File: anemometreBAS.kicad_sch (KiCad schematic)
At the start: 12 parts, among them J1 Conn_01x03_Male, J2 Conn_01x02_Male, J3 Conn_01x02_Male, J4 Conn_01x02_Male, J5 Conn_01x02_Male, U1 TP4056

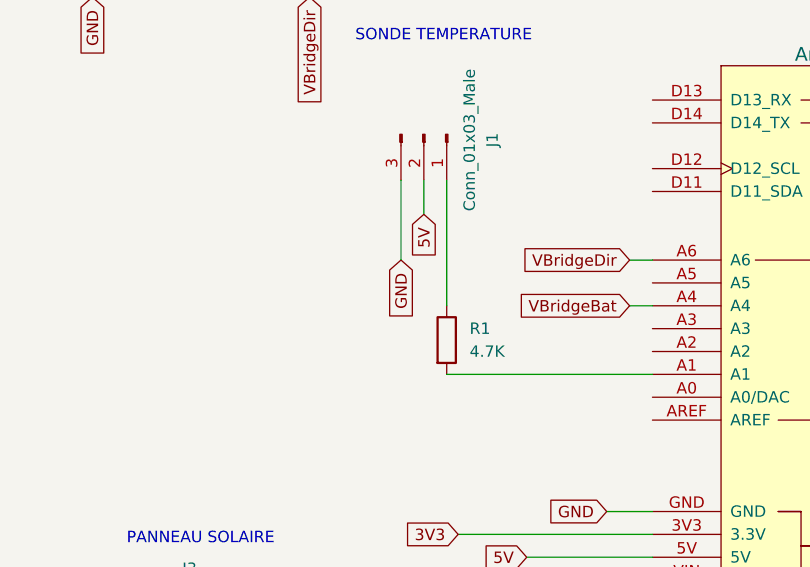
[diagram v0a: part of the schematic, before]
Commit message: fix error
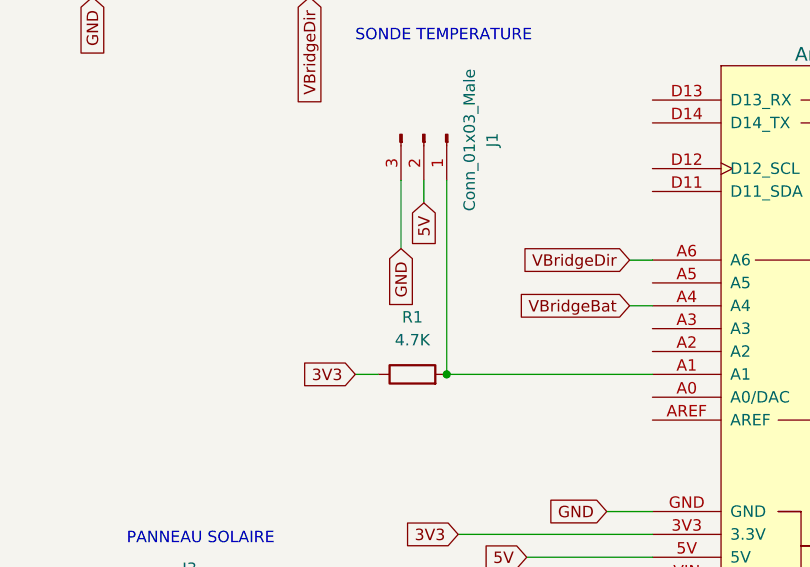
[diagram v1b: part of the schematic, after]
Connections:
- net 3V3: now also R1.1
- net at J1.1 (Pin_1): now also R1.2, XA1.A1; no longer R1.1
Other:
- moved on the sheet: R1
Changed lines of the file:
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@@
 (kicad_sch (version 20211123) (generator eeschema)
   (paper "A4")
+  (junction (at 100.33 86.36) (diameter 0) (color 0 0 0 0)
+  )
   (junction (at 34.29 76.2) (diameter 0) (color 0 0 0 0)
   )
@@
   (junction (at 199.39 55.88) (diameter 0) (color 0 0 0 0)
   )
+  (wire (pts (xy 90.17 86.36) (xy 92.71 86.36))
+    (stroke (width 0) (type default) (color 0 0 0 0))
+  )
+  (wire (pts (xy 199.39 55.88) (xy 208.28 55.88))
+    (stroke (width 0) (type default) (color 0 0 0 0))
+  )
+  (wire (pts (xy 76.2 113.03) (xy 83.82 113.03))
+    (stroke (width 0) (type default) (color 0 0 0 0))
+  )
+  (wire (pts (xy 34.29 60.96) (xy 34.29 66.04))
+    (stroke (width 0) (type default) (color 0 0 0 0))
+  )
+  (wire (pts (xy 205.74 58.42) (xy 208.28 58.42))
+    (stroke (width 0) (type default) (color 0 0 0 0))
+  )
+  (wire (pts (xy 34.29 76.2) (xy 38.1 76.2))
+    (stroke (width 0) (type default) (color 0 0 0 0))
+  )
+  (wire (pts (xy 118.11 109.22) (xy 123.19 109.22))
+    (stroke (width 0) (type default) (color 0 0 0 0))
+  )
+  (wire (pts (xy 34.29 86.36) (xy 34.29 91.44))
+    (stroke (width 0) (type default) (color 0 0 0 0))
+  )
+  (wire (pts (xy 101.6 104.14) (xy 123.19 104.14))
+    (stroke (width 0) (type default) (color 0 0 0 0))
+  )
+  (wire (pts (xy 76.2 115.57) (xy 83.82 115.57))
+    (stroke (width 0) (type default) (color 0 0 0 0))
+  )
+  (wire (pts (xy 120.65 78.74) (xy 123.19 78.74))
+    (stroke (width 0) (type default) (color 0 0 0 0))
+  )
+  (wire (pts (xy 80.01 125.73) (xy 83.82 125.73))
+    (stroke (width 0) (type default) (color 0 0 0 0))
+  )
+  (wire (pts (xy 97.79 64.77) (xy 97.79 67.31))
+    (stroke (width 0) (type default) (color 0 0 0 0))
+  )
+  (wire (pts (xy 120.65 73.66) (xy 123.19 73.66))
+    (stroke (width 0) (type default) (color 0 0 0 0))
+  )
+  (wire (pts (xy 189.23 55.88) (xy 199.39 55.88))
+    (stroke (width 0) (type default) (color 0 0 0 0))
+  )
+  (wire (pts (xy 60.96 40.64) (xy 60.96 44.45))
+    (stroke (width 0) (type default) (color 0 0 0 0))
+  )
+  (wire (pts (xy 199.39 40.64) (xy 199.39 48.26))
+    (stroke (width 0) (type default) (color 0 0 0 0))
+  )
+  (wire (pts (xy 72.39 128.27) (xy 83.82 128.27))
+    (stroke (width 0) (type default) (color 0 0 0 0))
+  )
+  (wire (pts (xy 109.22 106.68) (xy 123.19 106.68))
+    (stroke (width 0) (type default) (color 0 0 0 0))
+  )
+  (wire (pts (xy 85.09 40.64) (xy 85.09 38.1))
+    (stroke (width 0) (type default) (color 0 0 0 0))
+  )
+  (wire (pts (xy 95.25 64.77) (xy 95.25 72.39))
+    (stroke (width 0) (type default) (color 0 0 0 0))
+  )
+  (wire (pts (xy 60.96 120.65) (xy 83.82 120.65))
+    (stroke (width 0) (type default) (color 0 0 0 0))
+  )
+  (wire (pts (xy 118.11 101.6) (xy 123.19 101.6))
+    (stroke (width 0) (type default) (color 0 0 0 0))
+  )
+  (wire (pts (xy 85.09 40.64) (xy 85.09 44.45))
+    (stroke (width 0) (type default) (color 0 0 0 0))
+  )
+  (wire (pts (xy 60.96 118.11) (xy 83.82 118.11))
+    (stroke (width 0) (type default) (color 0 0 0 0))
+  )
+  (wire (pts (xy 34.29 73.66) (xy 34.29 76.2))
+    (stroke (width 0) (type default) (color 0 0 0 0))
+  )
+  (wire (pts (xy 34.29 76.2) (xy 34.29 78.74))
+    (stroke (width 0) (type default) (color 0 0 0 0))
+  )
+  (wire (pts (xy 63.5 40.64) (xy 85.09 40.64))
+    (stroke (width 0) (type default) (color 0 0 0 0))
+  )
+  (wire (pts (xy 85.09 25.4) (xy 85.09 30.48))
+    (stroke (width 0) (type default) (color 0 0 0 0))
+  )
+  (wire (pts (xy 100.33 64.77) (xy 100.33 86.36))
+    (stroke (width 0) (type default) (color 0 0 0 0))
+  )
   (wire (pts (xy 100.33 86.36) (xy 123.19 86.36))
-    (stroke (width 0) (type default) (color 0 0 0 0))
-  )
-  (wire (pts (xy 199.39 55.88) (xy 208.28 55.88))
-    (stroke (width 0) (type default) (color 0 0 0 0))
-  )
-  (wire (pts (xy 76.2 113.03) (xy 83.82 113.03))
-    (stroke (width 0) (type default) (color 0 0 0 0))
-  )
-  (wire (pts (xy 34.29 60.96) (xy 34.29 66.04))
-    (stroke (width 0) (type default) (color 0 0 0 0))
-  )
-  (wire (pts (xy 205.74 58.42) (xy 208.28 58.42))
-    (stroke (width 0) (type default) (color 0 0 0 0))
-  )
-  (wire (pts (xy 34.29 76.2) (xy 38.1 76.2))
-    (stroke (width 0) (type default) (color 0 0 0 0))
-  )
-  (wire (pts (xy 118.11 109.22) (xy 123.19 109.22))
-    (stroke (width 0) (type default) (color 0 0 0 0))
-  )
-  (wire (pts (xy 34.29 86.36) (xy 34.29 91.44))
-    (stroke (width 0) (type default) (color 0 0 0 0))
-  )
-  (wire (pts (xy 101.6 104.14) (xy 123.19 104.14))
-    (stroke (width 0) (type default) (color 0 0 0 0))
-  )
-  (wire (pts (xy 76.2 115.57) (xy 83.82 115.57))
-    (stroke (width 0) (type default) (color 0 0 0 0))
-  )
-  (wire (pts (xy 120.65 78.74) (xy 123.19 78.74))
-    (stroke (width 0) (type default) (color 0 0 0 0))
-  )
-  (wire (pts (xy 80.01 125.73) (xy 83.82 125.73))
-    (stroke (width 0) (type default) (color 0 0 0 0))
-  )
-  (wire (pts (xy 97.79 64.77) (xy 97.79 68.58))
-    (stroke (width 0) (type default) (color 0 0 0 0))
-  )
-  (wire (pts (xy 120.65 73.66) (xy 123.19 73.66))
-    (stroke (width 0) (type default) (color 0 0 0 0))
-  )
-  (wire (pts (xy 189.23 55.88) (xy 199.39 55.88))
-    (stroke (width 0) (type default) (color 0 0 0 0))
-  )
-  (wire (pts (xy 60.96 40.64) (xy 60.96 44.45))
-    (stroke (width 0) (type default) (color 0 0 0 0))
-  )
-  (wire (pts (xy 199.39 40.64) (xy 199.39 48.26))
-    (stroke (width 0) (type default) (color 0 0 0 0))
-  )
-  (wire (pts (xy 72.39 128.27) (xy 83.82 128.27))
-    (stroke (width 0) (type default) (color 0 0 0 0))
-  )
-  (wire (pts (xy 109.22 106.68) (xy 123.19 106.68))
-    (stroke (width 0) (type default) (color 0 0 0 0))
-  )
-  (wire (pts (xy 85.09 40.64) (xy 85.09 38.1))
-    (stroke (width 0) (type default) (color 0 0 0 0))
-  )
-  (wire (pts (xy 95.25 64.77) (xy 95.25 73.66))
-    (stroke (width 0) (type default) (color 0 0 0 0))
-  )
-  (wire (pts (xy 60.96 120.65) (xy 83.82 120.65))
-    (stroke (width 0) (type default) (color 0 0 0 0))
-  )
-  (wire (pts (xy 118.11 101.6) (xy 123.19 101.6))
-    (stroke (width 0) (type default) (color 0 0 0 0))
-  )
-  (wire (pts (xy 85.09 40.64) (xy 85.09 44.45))
-    (stroke (width 0) (type default) (color 0 0 0 0))
-  )
-  (wire (pts (xy 60.96 118.11) (xy 83.82 118.11))
-    (stroke (width 0) (type default) (color 0 0 0 0))
-  )
-  (wire (pts (xy 34.29 73.66) (xy 34.29 76.2))
-    (stroke (width 0) (type default) (color 0 0 0 0))
-  )
-  (wire (pts (xy 34.29 76.2) (xy 34.29 78.74))
-    (stroke (width 0) (type default) (color 0 0 0 0))
-  )
-  (wire (pts (xy 100.33 64.77) (xy 100.33 78.74))
-    (stroke (width 0) (type default) (color 0 0 0 0))
-  )
-  (wire (pts (xy 63.5 40.64) (xy 85.09 40.64))
-    (stroke (width 0) (type default) (color 0 0 0 0))
-  )
-  (wire (pts (xy 85.09 25.4) (xy 85.09 30.48))
     (stroke (width 0) (type default) (color 0 0 0 0))
   )
@@
     )
   )
+  (global_label "3V3" (shape input) (at 90.17 86.36 180) (fields_autoplaced)
+    (effects (font (size 1.27 1.27)) (justify right))
+    (property "Intersheet References" "${INTERSHEET_REFS}" (id 0) (at 84.2493 86.4394 0)
+      (effects (font (size 1.27 1.27)) (justify left) hide)
+    )
+  )
   (global_label "VIN" (shape input) (at 80.01 125.73 180) (fields_autoplaced)
     (effects (font (size 1.27 1.27)) (justify right))
@@
     )
   )
-  (global_label "5V" (shape input) (at 97.79 68.58 270) (fields_autoplaced)
-    (effects (font (size 1.27 1.27)) (justify right))
-    (property "Intersheet References" "${INTERSHEET_REFS}" (id 0) (at 97.8694 73.2912 90)
+  (global_label "5V" (shape input) (at 97.79 67.31 270) (fields_autoplaced)
+    (effects (font (size 1.27 1.27)) (justify right))
+    (property "Intersheet References" "${INTERSHEET_REFS}" (id 0) (at 97.8694 72.0212 90)
       (effects (font (size 1.27 1.27)) (justify left) hide)
     )
@@
     )
   )
-  (global_label "GND" (shape input) (at 95.25 73.66 270) (fields_autoplaced)
-    (effects (font (size 1.27 1.27)) (justify right))
-    (property "Intersheet References" "${INTERSHEET_REFS}" (id 0) (at 95.3294 79.9436 90)
+  (global_label "GND" (shape input) (at 95.25 72.39 270) (fields_autoplaced)
+    (effects (font (size 1.27 1.27)) (justify right))
+    (property "Intersheet References" "${INTERSHEET_REFS}" (id 0) (at 95.3294 78.6736 90)
       (effects (font (size 1.27 1.27)) (justify left) hide)
     )
@@
     (pin "2")
   )
-  (symbol (lib_id "Device:R") (at 100.33 82.55 0) (unit 1)
-    (in_bom yes) (on_board yes) (fields_autoplaced)
-    (property "Reference" "R1" (id 0) (at 102.87 81.2799 0)
-      (effects (font (size 1.27 1.27)) (justify left))
-    )
-    (property "Value" "4.7K" (id 1) (at 102.87 83.8199 0)
-      (effects (font (size 1.27 1.27)) (justify left))
-    )
-    (property "Footprint" "" (id 2) (at 98.552 82.55 90)
-      (effects (font (size 1.27 1.27)) hide)
-    )
-    (property "Datasheet" "~" (id 3) (at 100.33 82.55 0)
-      (effects (font (size 1.27 1.27)) hide)
-    )
+  (symbol (lib_id "Device:R") (at 96.52 86.36 90) (unit 1)
+    (in_bom yes) (on_board yes) (fields_autoplaced)
+    (property "Reference" "R1" (id 0) (at 96.52 80.01 90))
+    (property "Value" "4.7K" (id 1) (at 96.52 82.55 90))
+    (property "Footprint" "" (id 2) (at 96.52 88.138 90)
+      (effects (font (size 1.27 1.27)) hide)
+    )
+    (property "Datasheet" "~" (id 3) (at 96.52 86.36 0)
+      (effects (font (size 1.27 1.27)) hide)
+    )
